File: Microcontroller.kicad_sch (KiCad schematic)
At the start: 17 parts, among them IC3 W25Q128JVSIQ, IC4 ESP32-S3R8, Q1 40MHz

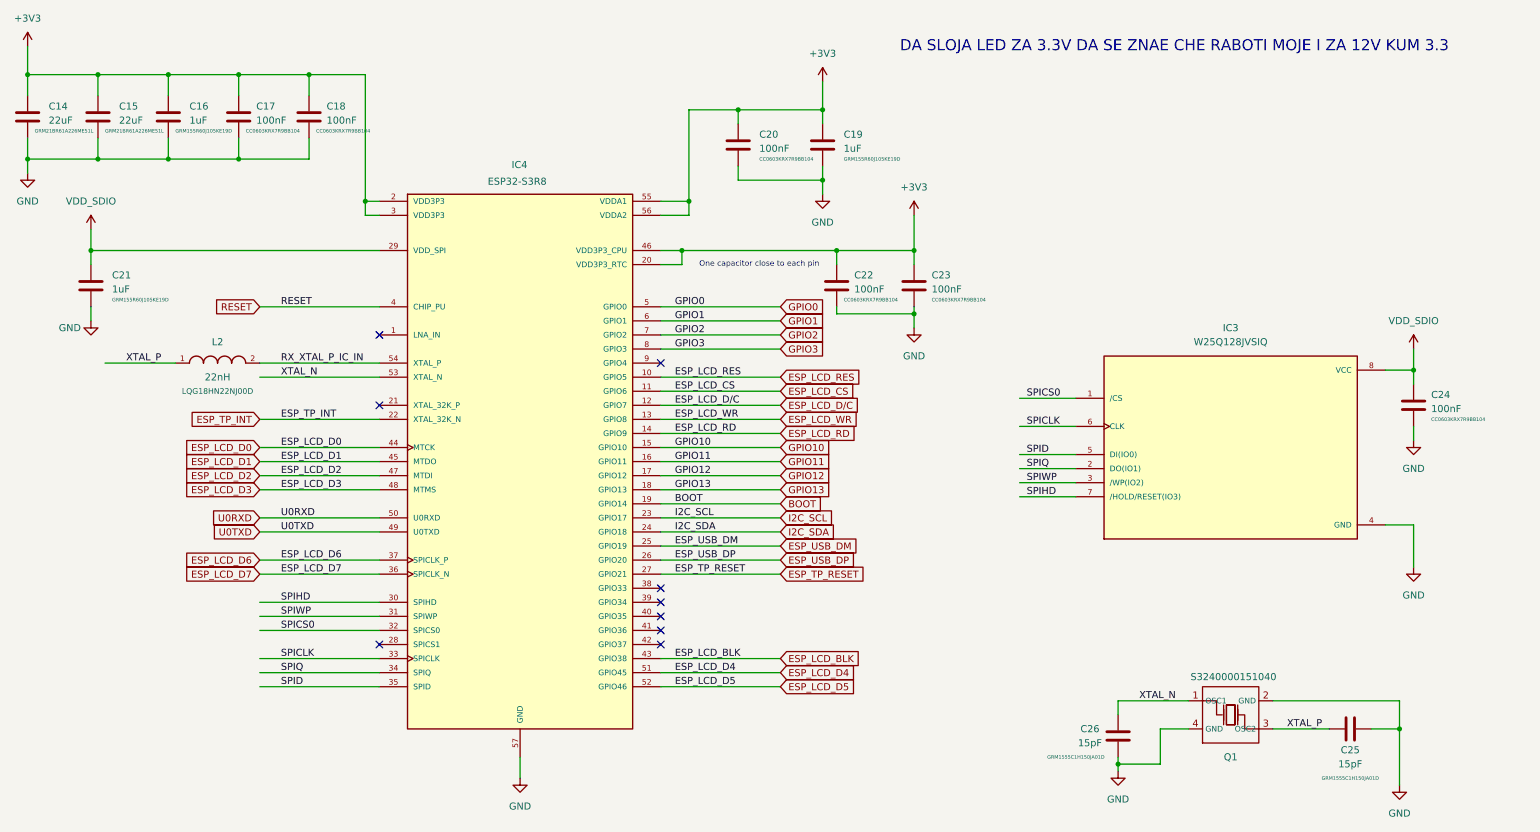
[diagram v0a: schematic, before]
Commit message: Changes to final schematic
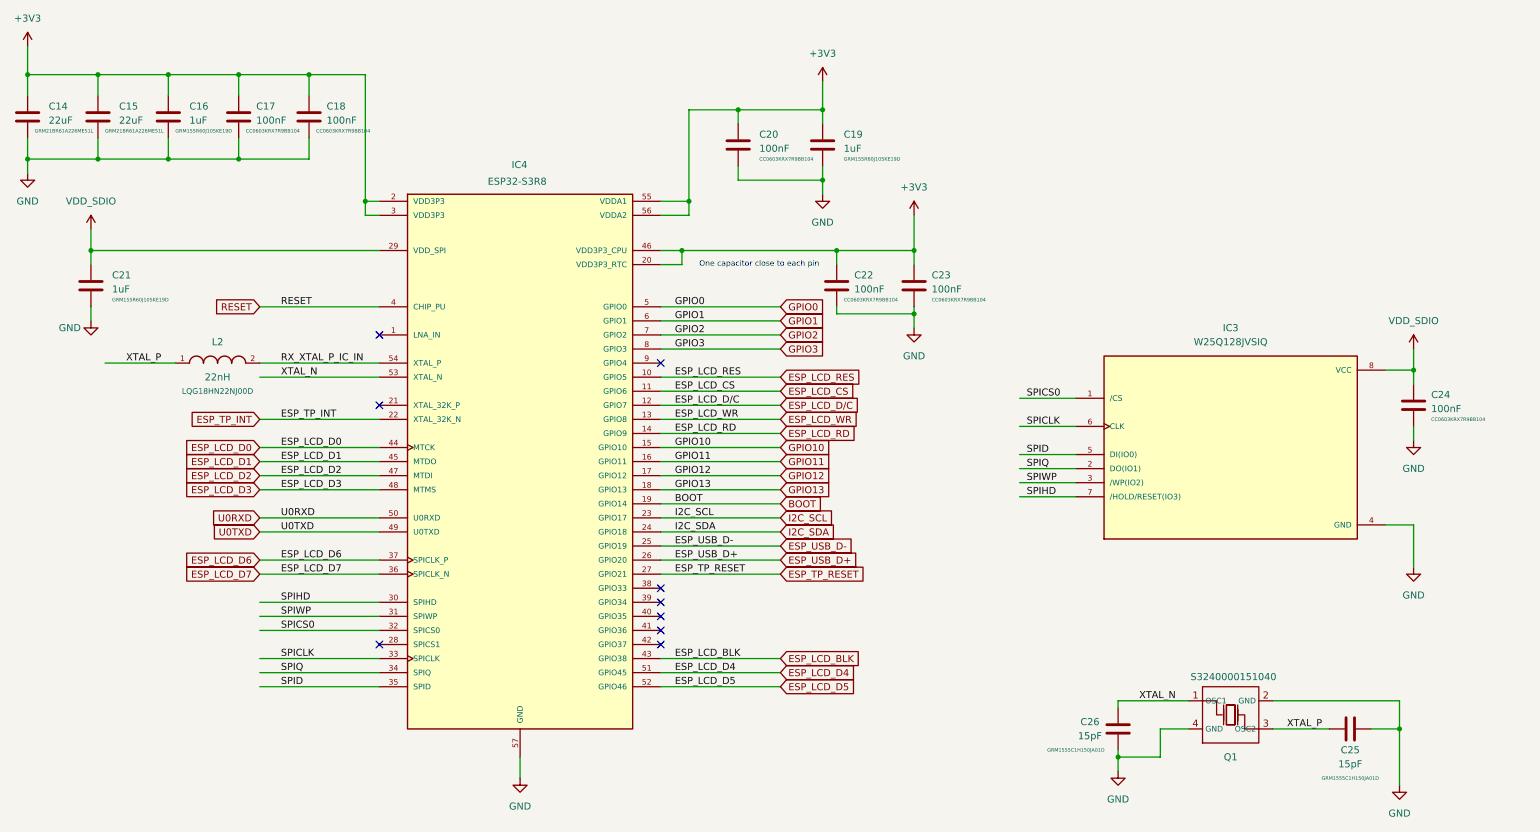
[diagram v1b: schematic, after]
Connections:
- net ESP_USB_DM renamed ESP_USB_D-
- net ESP_USB_DP renamed ESP_USB_D+
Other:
- note removed: "DA SLOJA LED ZA 3.3V DA SE ZNAE CHE RABOTI MOJE I ZA 12V KUM 3.3"
- moved on the sheet: C26
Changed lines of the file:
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@@
 	(generator_version "9.0")
 	(paper "A4")
-	(text "DA SLOJA LED ZA 3.3V DA SE ZNAE CHE RABOTI MOJE I ZA 12V KUM 3.3"
-		(exclude_from_sim no)
-		(at 224.79 24.13 0)
-		(effects
-			(font
-				(size 2 2)
-			)
-		)
-	)
 	(text "One capacitor close to each pin"
 		(exclude_from_sim no)
@@
 	)
 	(junction
-		(at 177.8 72.39)
+		(at 214.63 152.4)
 		(diameter 0)
 		(color 0 0 0 0)
 	)
 	(junction
-		(at 267.97 82.55)
+		(at 177.8 72.39)
 		(diameter 0)
 		(color 0 0 0 0)
 	)
 	(junction
-		(at 68.58 29.21)
+		(at 267.97 82.55)
 		(diameter 0)
 		(color 0 0 0 0)
 	)
 	(junction
-		(at 17.78 44.45)
+		(at 68.58 29.21)
 		(diameter 0)
 		(color 0 0 0 0)
 	)
 	(junction
-		(at 214.63 153.67)
+		(at 17.78 44.45)
 		(diameter 0)
 		(color 0 0 0 0)
@@
 	(wire
 		(pts
-			(xy 222.25 147.32) (xy 222.25 153.67)
+			(xy 222.25 147.32) (xy 222.25 152.4)
 		)
 		(stroke
@@
 	(wire
 		(pts
-			(xy 214.63 142.24) (xy 214.63 144.78)
+			(xy 214.63 142.24) (xy 214.63 143.51)
 		)
 		(stroke
@@
 	(wire
 		(pts
-			(xy 222.25 153.67) (xy 214.63 153.67)
-		)
-		(stroke
-			(width 0)
-			(type default)
-		)
-	)
-	(wire
-		(pts
-			(xy 214.63 153.67) (xy 214.63 154.94)
+			(xy 222.25 152.4) (xy 214.63 152.4)
 		)
 		(stroke
@@
 	(wire
 		(pts
+			(xy 214.63 152.4) (xy 214.63 154.94)
+		)
+		(stroke
+			(width 0)
+			(type default)
+		)
+	)
+	(wire
+		(pts
 			(xy 30.48 40.64) (xy 30.48 44.45)
 		)
@@
 	(wire
 		(pts
-			(xy 214.63 152.4) (xy 214.63 153.67)
+			(xy 214.63 151.13) (xy 214.63 152.4)
 		)
 		(stroke
@@
 		)
 	)
-	(label "ESP_USB_DM"
+	(label "ESP_USB_D-"
 		(at 134.62 114.3 0)
 		(effects
@@
 		)
 	)
-	(label "ESP_USB_DP"
+	(label "ESP_USB_D+"
 		(at 134.62 116.84 0)
 		(effects
@@
 		)
 	)
-	(global_label "ESP_USB_DM"
+	(global_label "ESP_USB_D-"
 		(shape input)
 		(at 153.67 114.3 0)
@@
 		)
 		(property "Intersheetrefs" "${INTERSHEET_REFS}"
-			(at 168.7503 114.3 0)
+			(at 168.8713 114.3 0)
 			(effects
 				(font
@@
 		)
 	)
-	(global_label "ESP_USB_DP"
+	(global_label "ESP_USB_D+"
 		(shape input)
 		(at 153.67 116.84 0)
@@
 		)
 		(property "Intersheetrefs" "${INTERSHEET_REFS}"
-			(at 168.5689 116.84 0)
+			(at 168.8713 116.84 0)
 			(effects
 				(font
@@
 	(symbol
 		(lib_id "Project Capacitors:GRM1555C1H150JA01D")
-		(at 214.63 148.59 0)
+		(at 214.63 147.32 0)
 		(mirror y)
 		(unit 1)
@@
 		(dnp no)
 		(property "Reference" "C26"
-			(at 209.55 147.32 0)
+			(at 209.55 146.05 0)
 			(effects
 				(font
@@
 		)
 		(property "Value" "15pF"
-			(at 209.55 149.86 0)
+			(at 209.55 148.59 0)
 			(effects
 				(font
@@
 		)
 		(property "Footprint" "GRM1555C1H150JA01D:CAPC1005X55N"
-			(at 213.6648 152.4 0)
+			(at 213.6648 151.13 0)
 			(effects
 				(font
@@
 		)
 		(property "Datasheet" "~"
-			(at 214.63 148.59 0)
+			(at 214.63 147.32 0)
 			(effects
 				(font
@@
 		)
 		(property "Description" "Unpolarized capacitor"
-			(at 214.63 148.59 0)
+			(at 214.63 147.32 0)
 			(effects
 				(font
@@
 		)
 		(property "Footprint Name" "GRM1555C1H150JA01D"
-			(at 207.01 152.4 0)
+			(at 207.01 151.13 0)
 			(effects
 				(font
